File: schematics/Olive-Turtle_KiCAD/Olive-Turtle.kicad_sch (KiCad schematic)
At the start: 11 parts, among them IC1 ENS160-BGLT, U1 ESP32-DEVKITC-32U

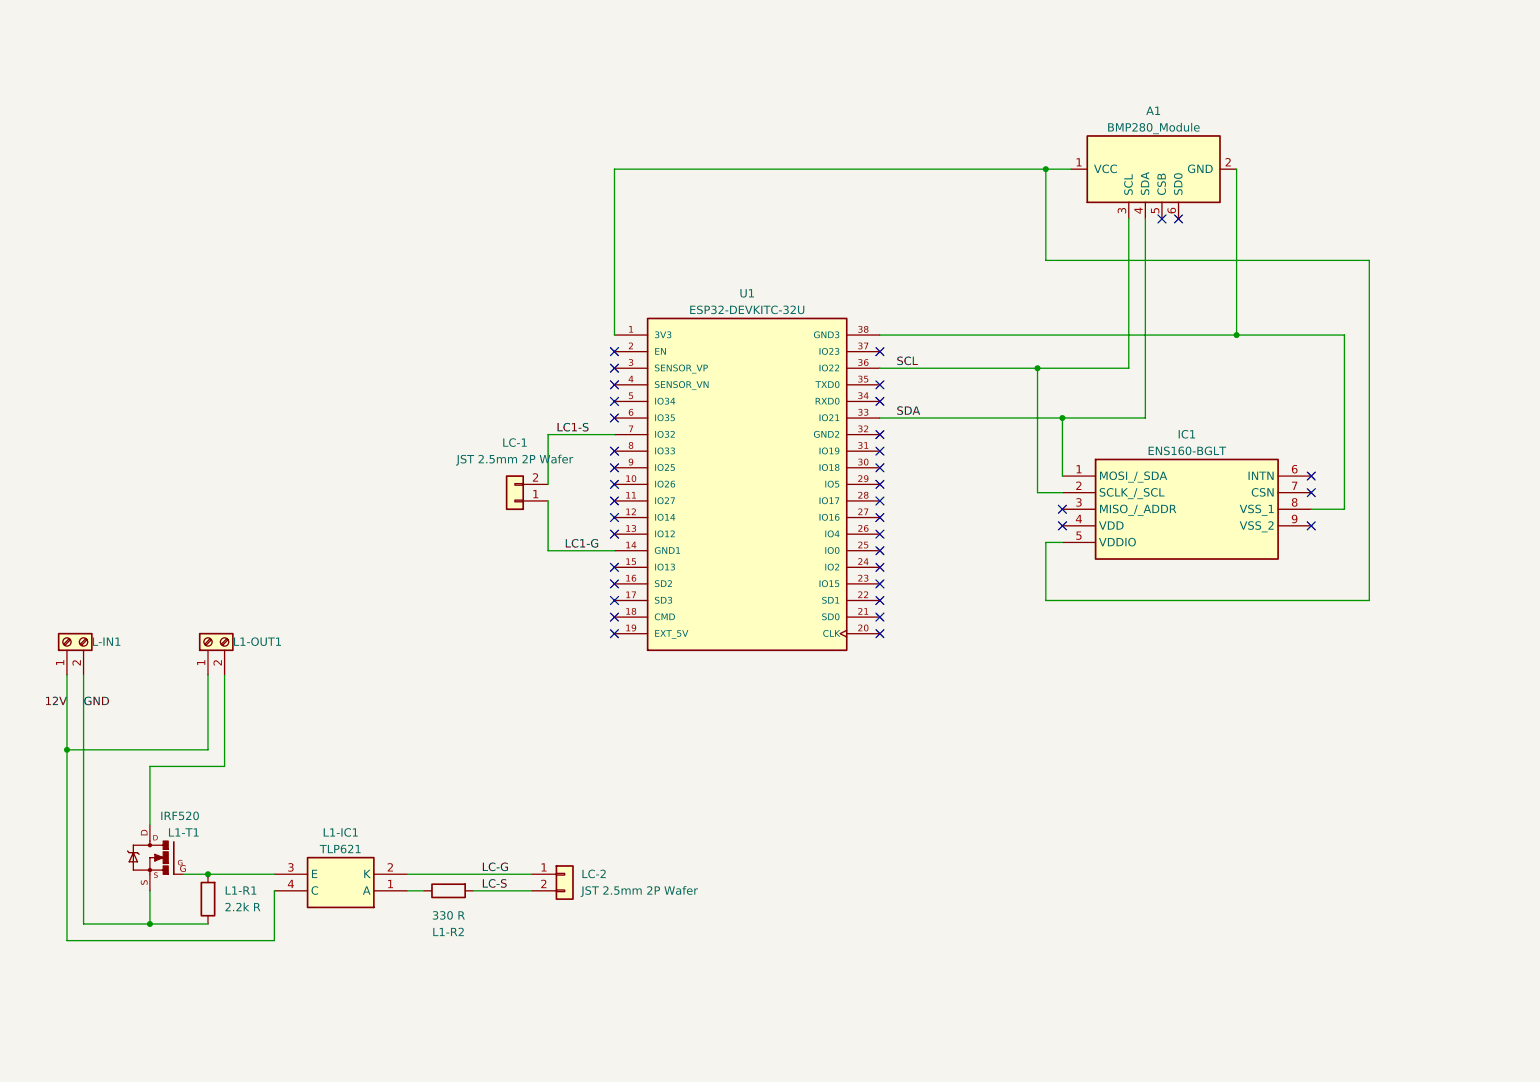
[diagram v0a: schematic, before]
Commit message: [develop] ProtoBoards for all other boards + refactor sch
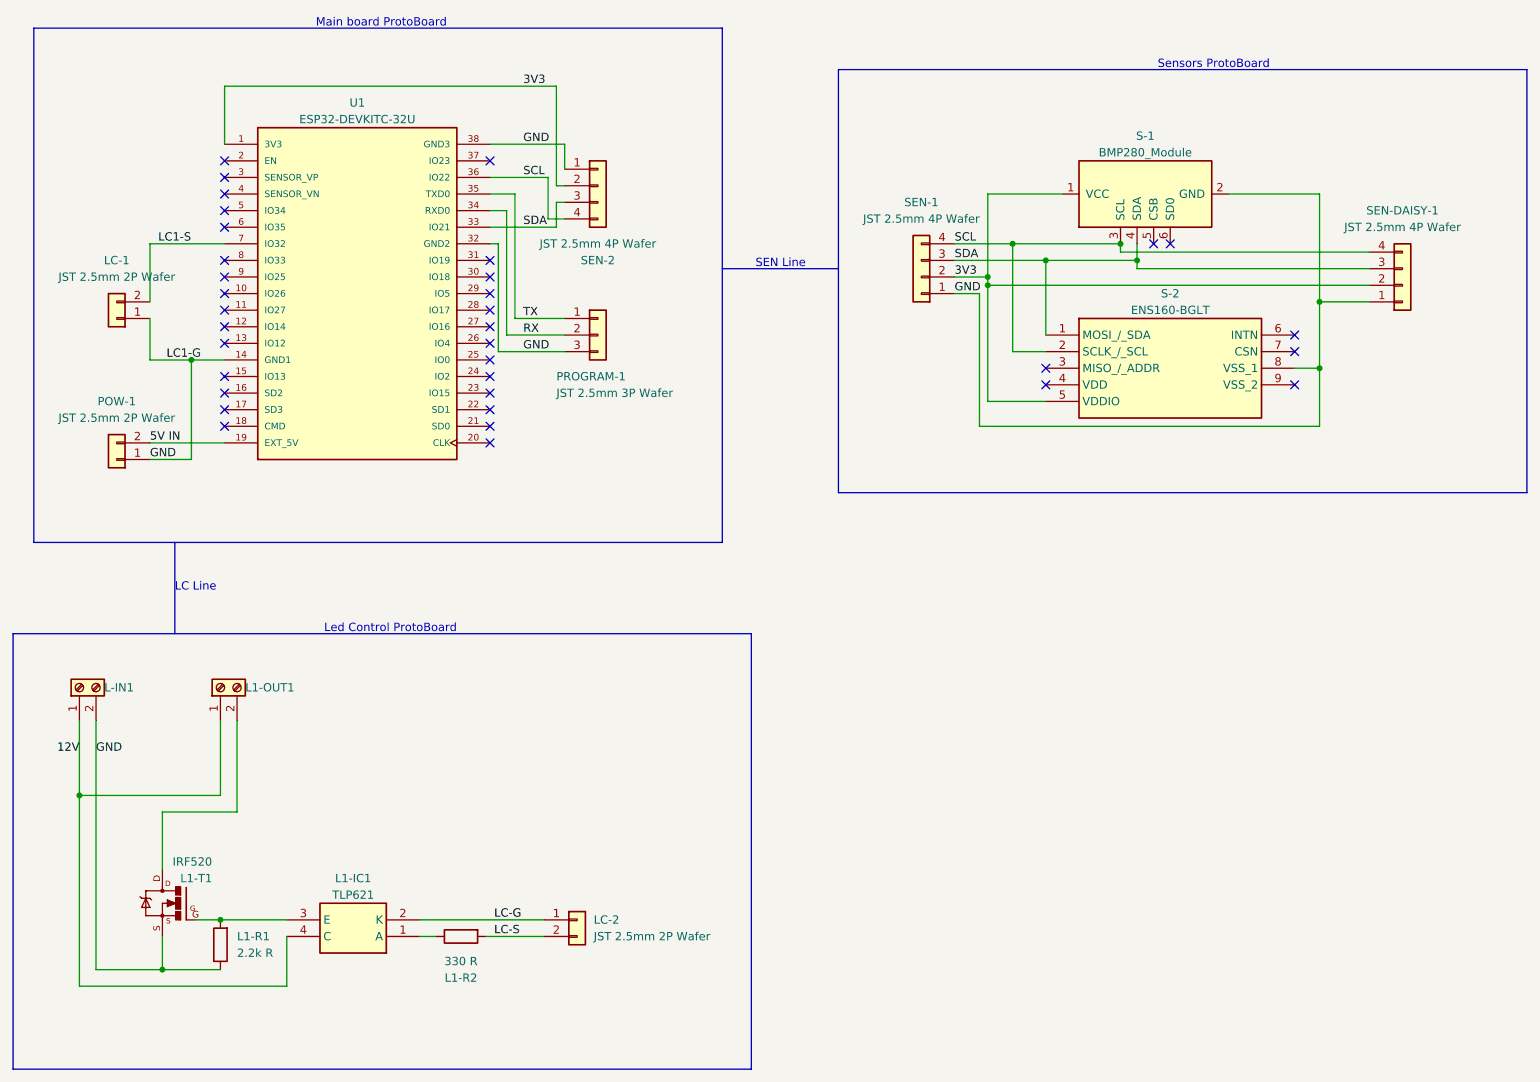
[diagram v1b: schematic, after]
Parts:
- added POW-1: JST 2.5mm 2P Wafer, Connector_JST:JST_EH_B2B-EH-A_1x02_P2.50mm_Vertical, symbol Connector_Generic:Conn_01x02
- added PROGRAM-1: JST 2.5mm 3P Wafer, symbol Connector_Generic:Conn_01x03
- added SEN-1, SEN-2, SEN-DAISY-1: JST 2.5mm 4P Wafer, symbol Connector_Generic:Conn_01x04
- renumbered A1 to S-1, IC1 to S-2
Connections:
- net LC1-G is gone; now on net GND: LC-1.1 (Pin_1), U1.14 (GND1)
- net GND: now also S-1.2 (GND), S-2.8 (VSS_1), U1.32 (GND2), U1.38 (GND3), POW-1.1 (Pin_1), PROGRAM-1.3 (Pin_3), SEN-1.1 (Pin_1), SEN-2.1 (Pin_1), SEN-DAISY-1.1 (Pin_1)
- net SCL: now also SEN-1.4 (Pin_4), SEN-2.4 (Pin_4), SEN-DAISY-1.4 (Pin_4)
- net SDA: now also SEN-1.3 (Pin_3), SEN-2.3 (Pin_3), SEN-DAISY-1.3 (Pin_3)
- net 3V3: now reaches S-1.1 (VCC), S-2.5 (VDDIO), U1.1 (3V3)
- net 3V3: now also SEN-1.2 (Pin_2), SEN-2.2 (Pin_2), SEN-DAISY-1.2 (Pin_2)
- net 5V IN: now reaches U1.19 (EXT_5V)
- net 5V IN: now also POW-1.2 (Pin_2)
- net RX: now reaches U1.34 (RXD0)
- net RX: now also PROGRAM-1.2 (Pin_2)
- net TX: now reaches U1.35 (TXD0)
- net TX: now also PROGRAM-1.1 (Pin_1)
- no-connect marks 39 -> 35
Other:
- note added: "LC Line"
- note added: "Led Control ProtoBoard"
- note added: "Main board ProtoBoard"
- note added: "SEN Line"
- note added: "Sensors ProtoBoard"
- moved on the sheet: L-IN1, L1-IC1, L1-OUT1, L1-R1, L1-R2, L1-T1, LC-1, LC-2, S-1, S-2, U1
